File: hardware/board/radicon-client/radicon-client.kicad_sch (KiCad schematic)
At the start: 7 parts, among them J1 PIN, Q1 NMOS, U1 TWE-L-DP-W

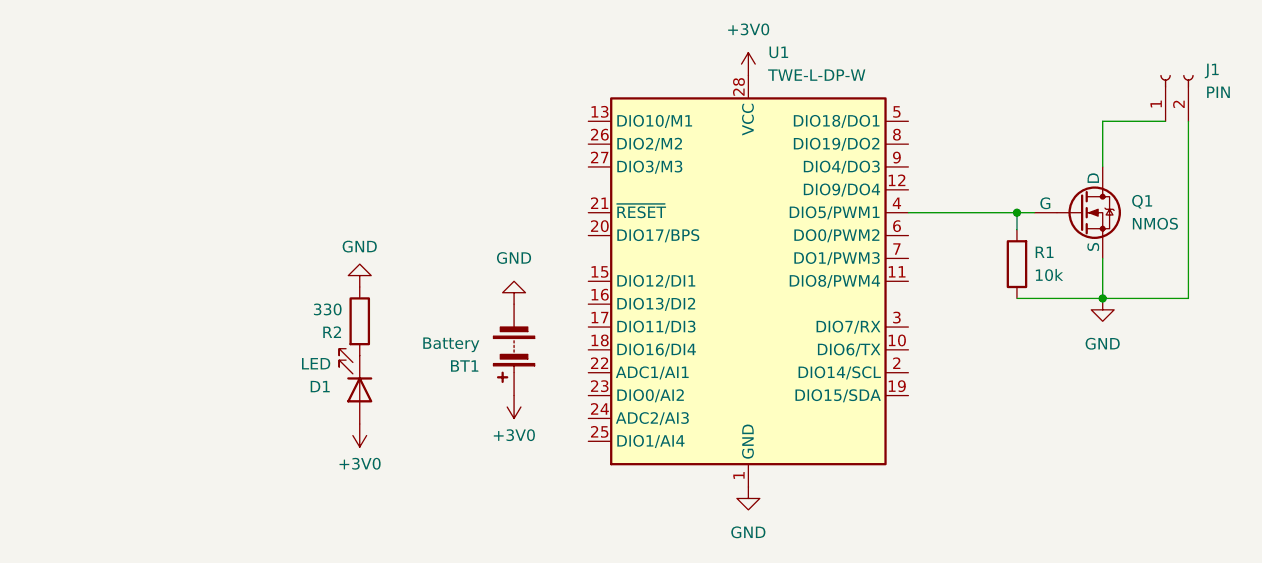
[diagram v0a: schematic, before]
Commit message: update board
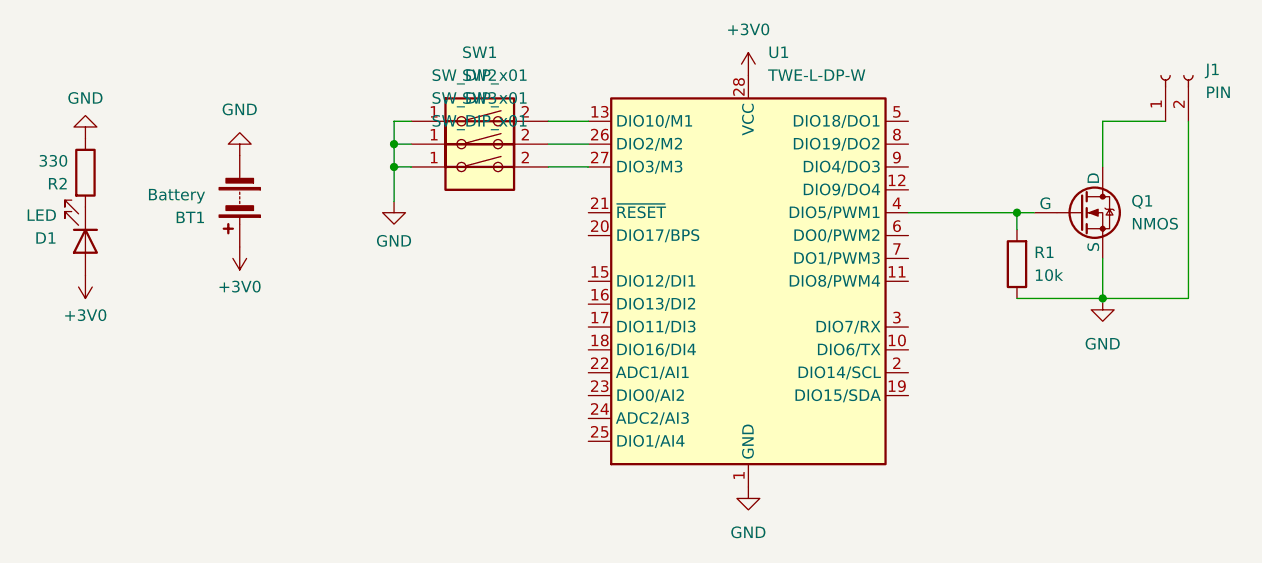
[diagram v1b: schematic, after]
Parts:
- added SW1, SW2, SW3: SW_DIP_x01, Jumper:SolderJumper-2_P1.3mm_Open_TrianglePad1.0x1.5mm, symbol Switch:SW_DIP_x01
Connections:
- net GND: now also SW1.1, SW2.1, SW3.1
- net at U1.13 (DIO10/M1): now also SW1.2
- net at U1.26 (DIO2/M2): now also SW2.2
- net at U1.27 (DIO3/M3): now also SW3.2
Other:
- moved on the sheet: BT1, D1, R2
